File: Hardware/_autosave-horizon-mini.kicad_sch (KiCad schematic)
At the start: 77 parts, among them J2 Conn_01x02_Pin, J3 Micro_SD_Card_Det1, J7 USB_C_Receptacle_USB2.0_16P, J8 Conn_02x03_Counter_Clockwise, Q1 BSS138, Q10 DMG2301L, U1 TPS82130, U16 AP2112K-3.3, U2 TPS61092, U3 LTC4412xS6, U5 ATSAMD21G18A-A, U6 NAND, U7 LPS22HB, U9 LSM6DS3

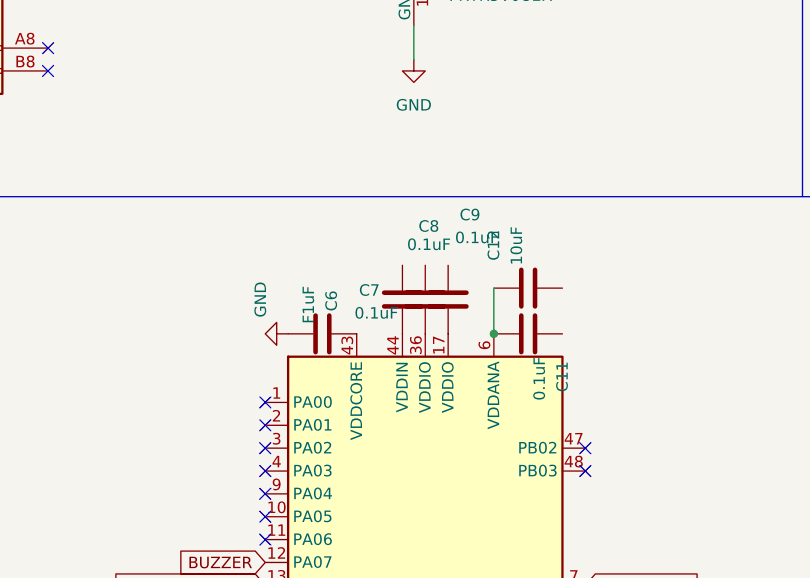
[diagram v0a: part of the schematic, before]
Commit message: please liam fix decop caps
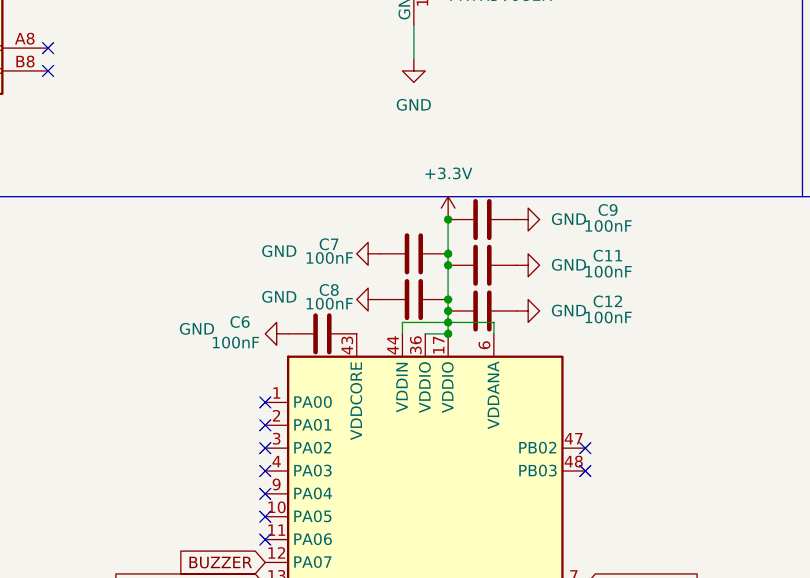
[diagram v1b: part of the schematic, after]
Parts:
- C11, C7, C8, C9: value 0.1uF -> 100nF
- C12: value 10uF -> 100nF
- C6: value F1uF -> 100nF
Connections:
- net +3.3V: now also C11.2, C12.2, C7.2, C8.2, C9.2, U5.17 (VDDIO), U5.36 (VDDIO), U5.44 (VDDIN), U5.6 (VDDANA)
- net GND: now also C11.1, C12.1, C6.1, C7.1, C8.1, C9.1; no longer C6.2
- net at U5.43 (VDDCORE): now also C6.2; no longer C6.1
